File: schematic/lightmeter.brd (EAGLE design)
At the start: 27.9 x 52.1 mm, 80 parts, among them IC2 MCP73831/OT, J1 AVR_SPI_PRG_6NS, Q1 NCHANNELMOSFET, Q10 PCHANNELMOSFET, Q11 NCHANNELMOSFET, Q12 NCHANNELMOSFET, Q13 NCHANNELMOSFET, Q14 NCHANNELMOSFET, Q16 NCHANNELMOSFET, Q2 PCHANNELMOSFET, Q3 NCHANNELMOSFET, Q4 PCHANNELMOSFET, Q5 NCHANNELMOSFET, Q6 PCHANNELMOSFET, Q7 NCHANNELMOSFET, Q8 PCHANNELMOSFET, Q9 PCHANNELMOSFET

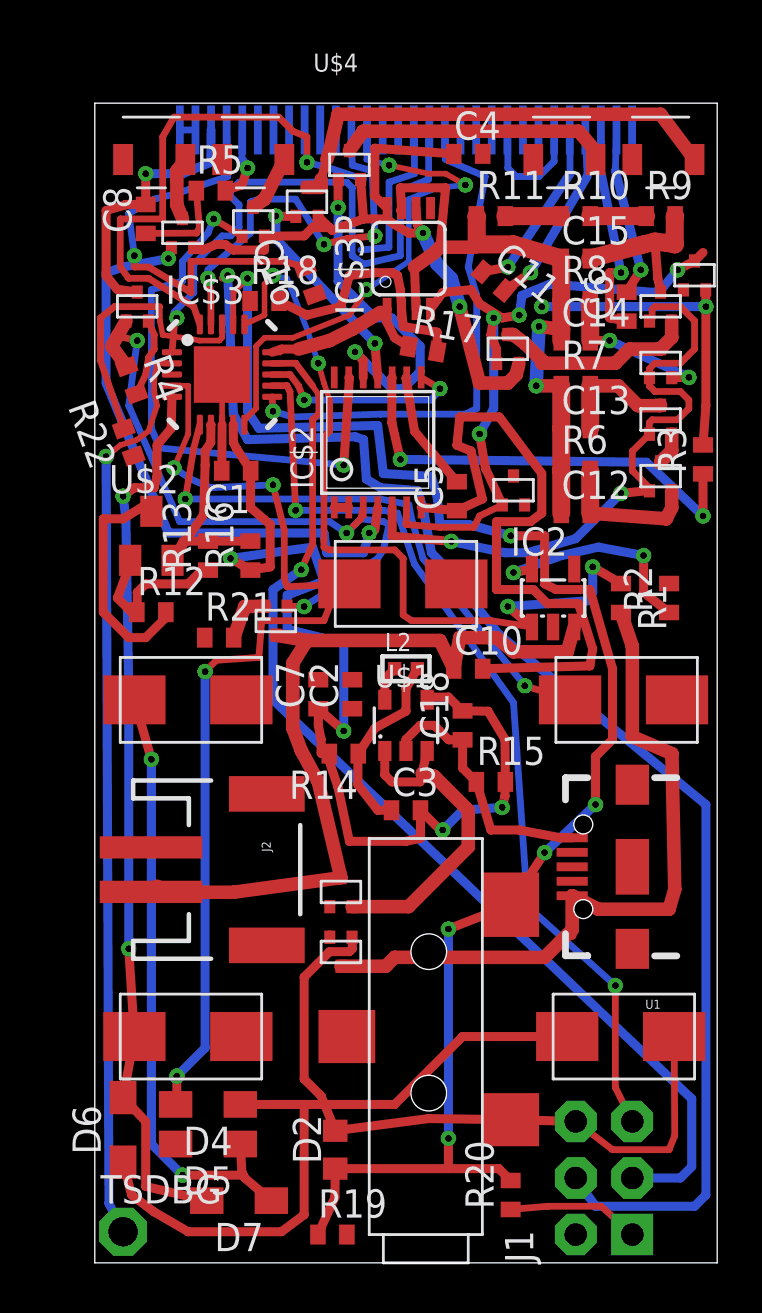
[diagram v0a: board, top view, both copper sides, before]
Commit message: More work on layout.
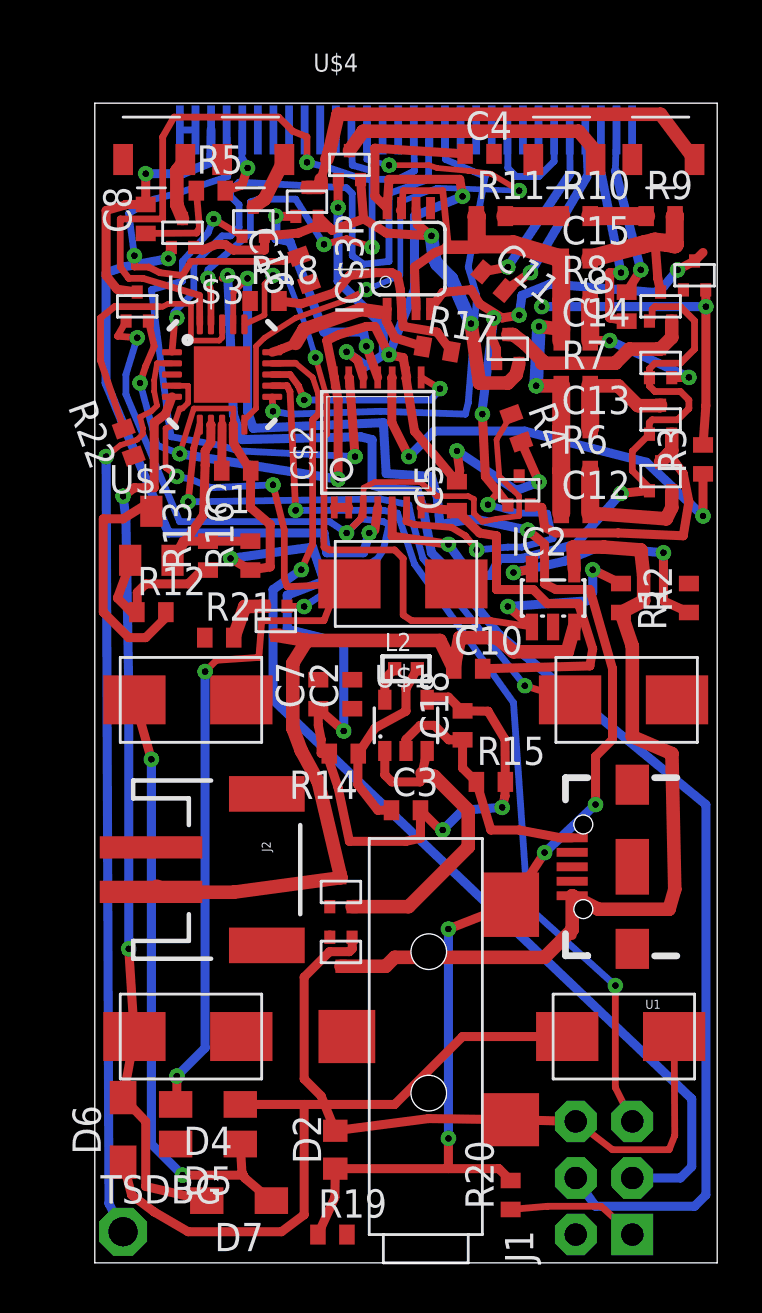
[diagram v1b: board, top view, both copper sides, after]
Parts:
- moved R4 17.4 mm to (17.7, 37.5)
- moved R2 0.89 mm to (25.4, 29.8)
- moved R17 0.63 mm to (14.1, 41.0)
- moved C16 0.57 mm to (8.13, 44.6)
- moved C4 0.51 mm to (16.0, 49.8)
- moved Q6 0.25 mm to (17.8, 34.9)
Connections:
- net N$22: now also Q6.P$2
- net N$26: now also Q6.P$3
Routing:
- net VREG: track 64.1 -> 113.0 mm, vias 4 -> 11
- net GND: track 107.9 -> 92.9 mm
- net SCRPWR: track 29.6 -> 42.2 mm
- net N$22: track 1.45 -> 13.1 mm
- net VUSB: track 33.5 -> 41.0 mm
- net STG$2: track 16.4 -> 23.2 mm, vias 2 -> 4
- net SCRCLK: track 23.4 -> 28.2 mm
- net DIODESW$3: track 15.8 -> 12.2 mm
- net SCRDC: track 31.0 -> 28.3 mm
- net N$12: track 18.7 -> 17.1 mm
- net STG$1: track 29.4 -> 30.7 mm
- net N$5: track 10.0 -> 11.2 mm
- net DIODESW$4: track 9.92 -> 10.8 mm
- net DIODESW$2: track 25.7 -> 24.8 mm
- net PBI$1: track 45.5 -> 46.3 mm
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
